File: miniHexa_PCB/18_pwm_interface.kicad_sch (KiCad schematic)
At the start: 22 parts, among them U5 PCA9685BS

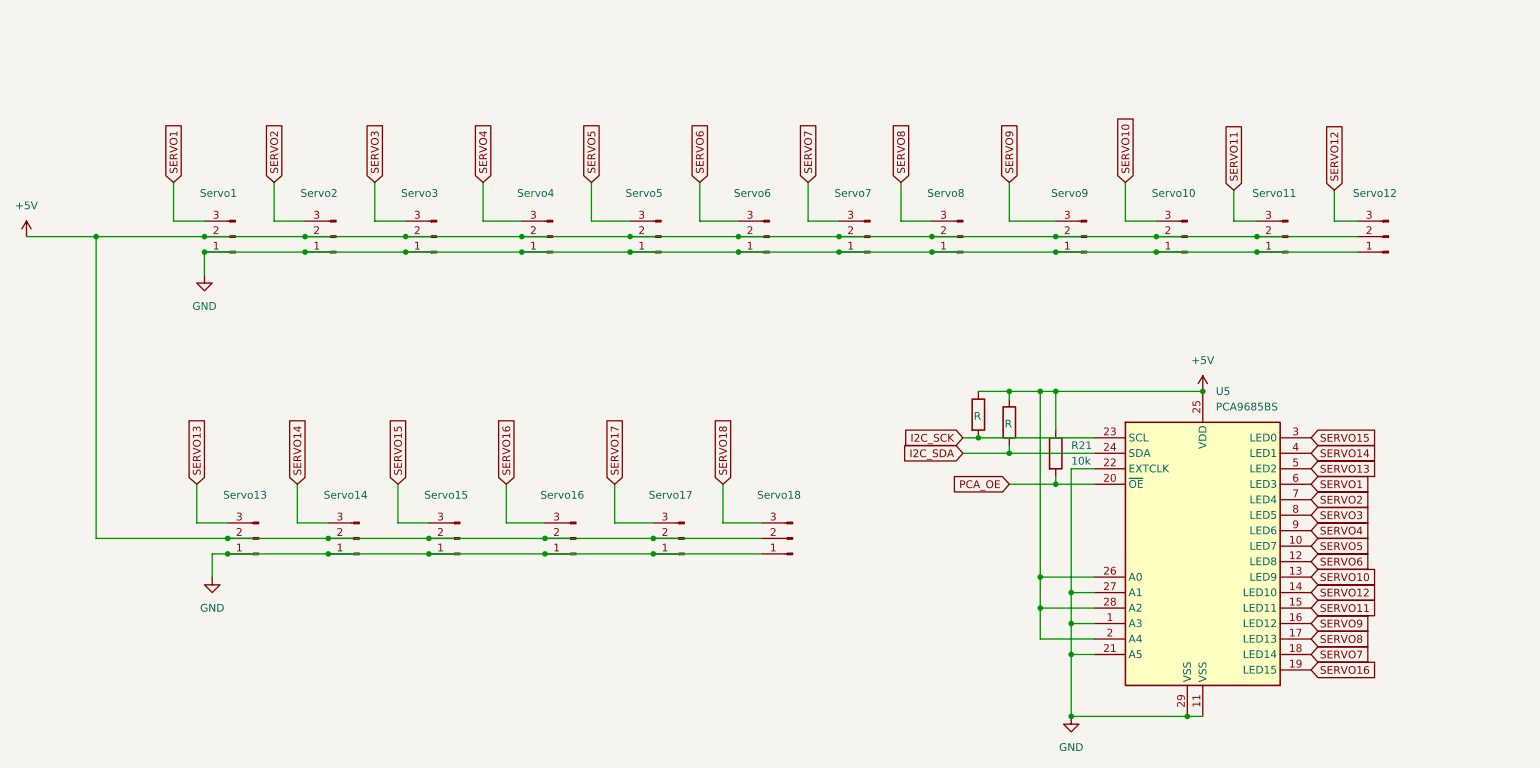
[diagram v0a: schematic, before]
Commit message: start of version 2.0
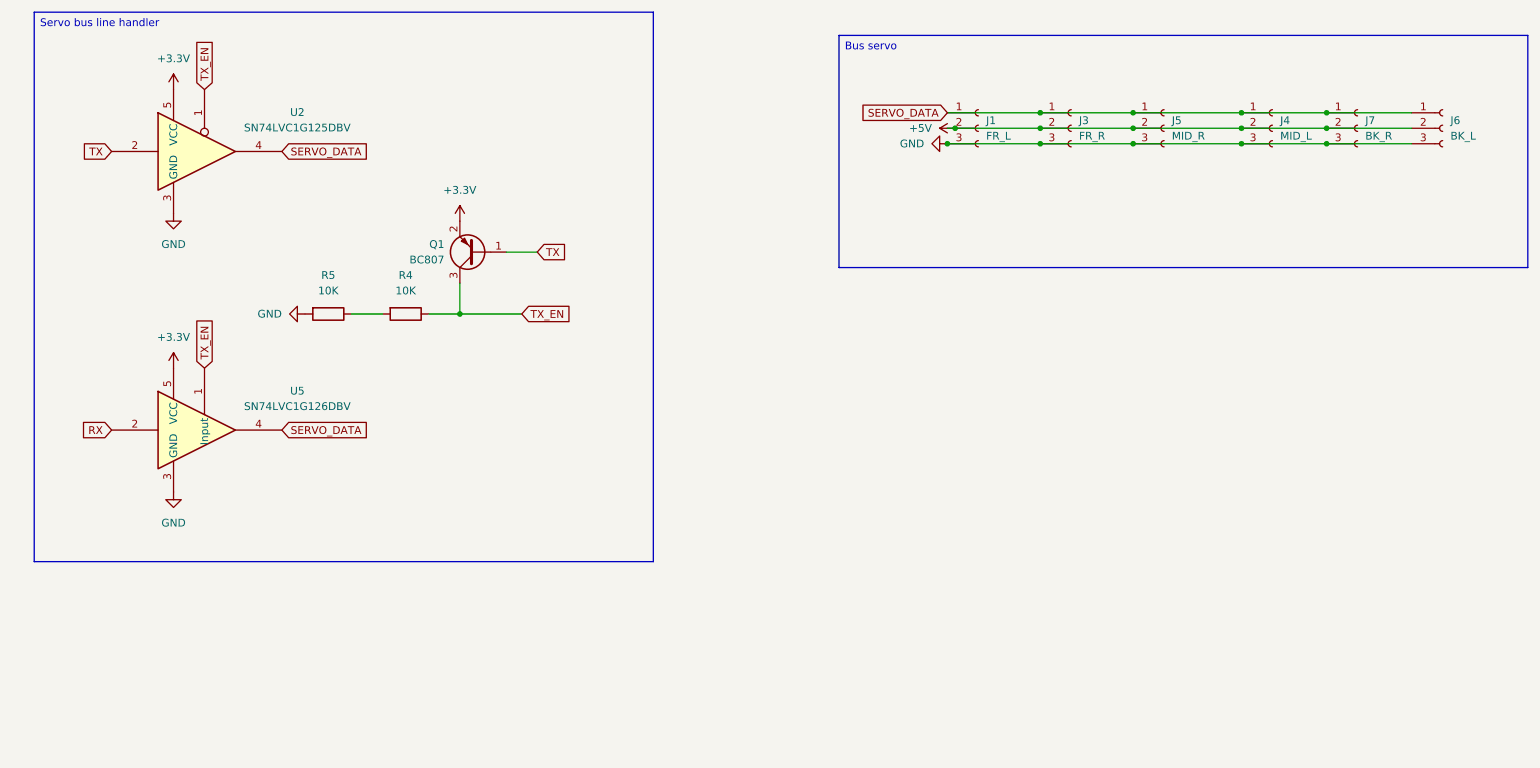
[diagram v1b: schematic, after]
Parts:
- removed R19: R, Resistor_SMD:R_0603_1608Metric, symbol Device:R
- removed R20: R, Resistor_SMD:R_0402_1005Metric, symbol Device:R
- removed R21: 10k, Resistor_SMD:R_0402_1005Metric, symbol Device:R
- removed Servo1, Servo10, Servo11, Servo12, Servo13, Servo14, Servo15, Servo16, Servo17, Servo18, Servo2, Servo3, Servo4, Servo5, Servo6, Servo7, Servo8, Servo9: Conn_01x03_Pin, Connector_JST:JST_XH_B3B-XH-AM_1x03_P2.50mm_Vertical, symbol Connector:Conn_01x03_Pin
- removed U5: PCA9685BS, Package_DFN_QFN:QFN-28-1EP_6x6mm_P0.65mm_EP4.25x4.25mm, symbol Driver_LED:PCA9685BS
- added J1: FR_L, Connector_JST:JST_XH_S3B-XH-A-1_1x03_P2.50mm_Horizontal, symbol Connector:Conn_01x03_Socket
- added J3: FR_R, Connector_JST:JST_XH_S3B-XH-A-1_1x03_P2.50mm_Horizontal, symbol Connector:Conn_01x03_Socket
- added J4: MID_L, Connector_JST:JST_XH_S3B-XH-A-1_1x03_P2.50mm_Horizontal, symbol Connector:Conn_01x03_Socket
- added J5: MID_R, Connector_JST:JST_XH_S3B-XH-A-1_1x03_P2.50mm_Horizontal, symbol Connector:Conn_01x03_Socket
- added J6: BK_L, Connector_JST:JST_XH_S3B-XH-A-1_1x03_P2.50mm_Horizontal, symbol Connector:Conn_01x03_Socket
- added J7: BK_R, Connector_JST:JST_XH_S3B-XH-A-1_1x03_P2.50mm_Horizontal, symbol Connector:Conn_01x03_Socket
- added Q1: BC807, Package_TO_SOT_SMD:SOT-23, symbol Transistor_BJT:BC807
- added R4, R5: 10K, symbol Device:R
- added U2: SN74LVC1G125DBV, Package_TO_SOT_SMD:SOT-23-5, symbol 74xGxx:SN74LVC1G125DBV
- added U5: SN74LVC1G126DBV, Package_TO_SOT_SMD:SOT-23-5, symbol 74xGxx:SN74LVC1G125DBV
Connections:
- net +5V: now also J1.2 (Pin_2), J3.2 (Pin_2), J4.2 (Pin_2), J5.2 (Pin_2), J6.2 (Pin_2), J7.2 (Pin_2)
- net GND: now also J1.3 (Pin_3), J3.3 (Pin_3), J4.3 (Pin_3), J5.3 (Pin_3), J6.3 (Pin_3), J7.3 (Pin_3), R5.2, U2.3 (GND), U5.3 (GND)
- new net: R4.2, R5.1
- new net +3.3V: Q1.2 (E), U2.5 (VCC), U5.5 (VCC)
- new net RX: U5.2
- new net SERVO_DATA: J1.1 (Pin_1), J3.1 (Pin_1), J4.1 (Pin_1), J5.1 (Pin_1), J6.1 (Pin_1), J7.1 (Pin_1), U2.4, U5.4
- new net TX: Q1.1 (B), U2.2
- new net TX_EN: Q1.3 (C), R4.1, U2.1, U5.1 (Input)
